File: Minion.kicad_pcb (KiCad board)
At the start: 2 copper layers, 60 x 60 mm, 70 parts, among them J1 USB_C_Receptacle_USB2.0_16P, J2 USB_A, J3 473092651, J4 PJ-320D-A, Q1 AO3401A, SW1 SW_Push, SW2 SW_Push, SW3 SW_Push, SW4 RotaryEncoder, SW5 SW_Push, SW6 SW_Push, U1 ESP32-S3-WROOM-1, U2 AMS1117-3.3, U3 FE1.1s, U4 ADXL343, U5 CH376T, U6 MCP73831-2-MC, U7 PCM5102A, Y1 12MHz, Y2 12MHz

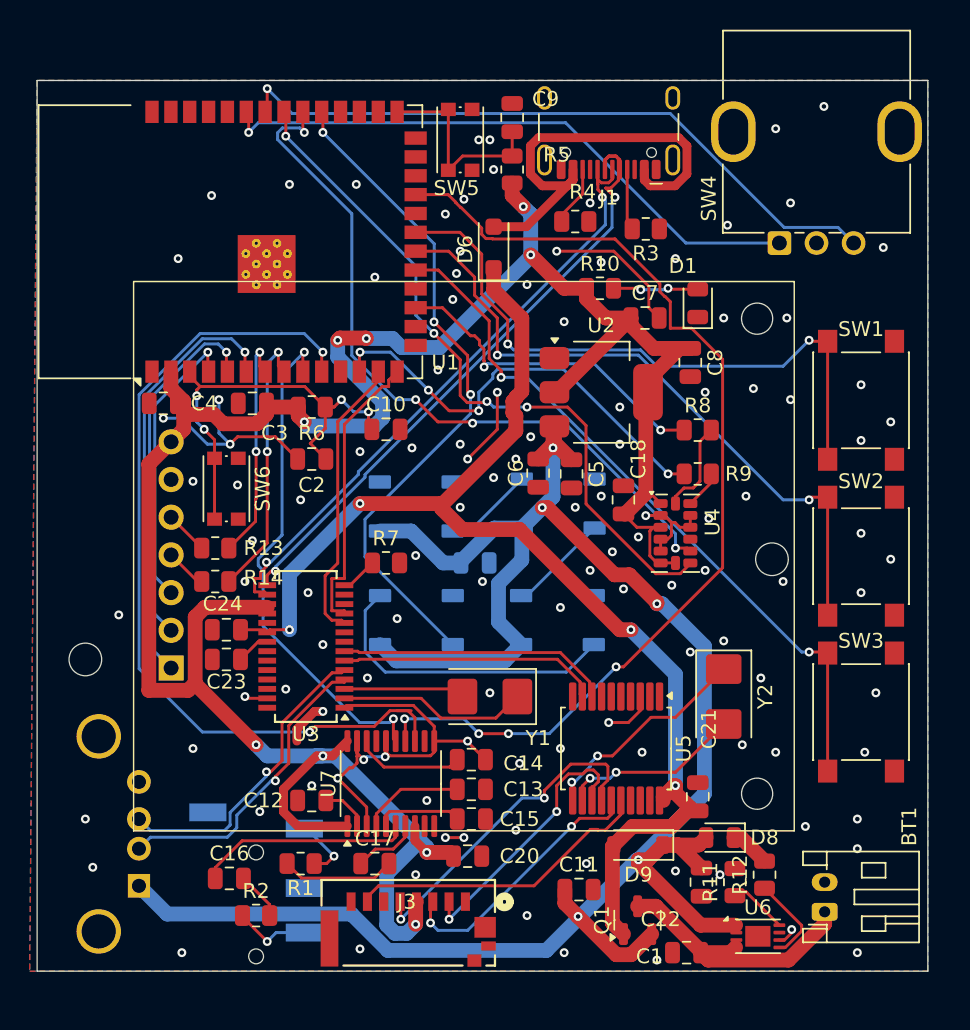
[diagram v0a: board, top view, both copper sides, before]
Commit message: Finished PCB!
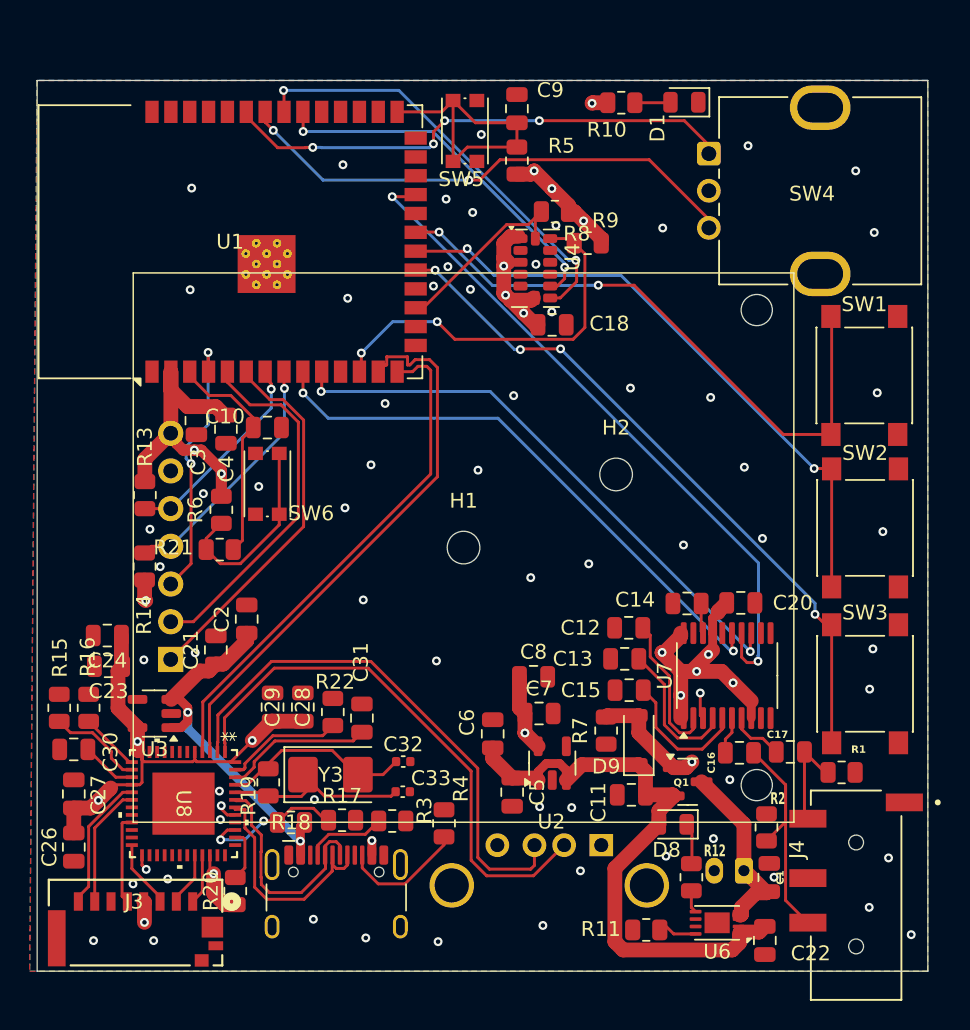
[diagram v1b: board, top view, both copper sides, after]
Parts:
- removed C19: 4.7uF, Capacitor_SMD:C_0805_2012Metric
- removed D2, D3, D4, D5: WS2812B, LED_SMD:LED_WS2812B_PLCC4_5.0x5.0mm_P3.2mm
- removed D6: S-LMBR340FT1G, Diode_SMD:D_SOD-123F
- removed DISPLAY_SSD1351: Conn_01x07_Socket, Connector_PinHeader_2.54mm:SSD_1351
- removed U5: CH376T, Package_SO:SSOP-20_5.3x7.2mm_P0.65mm
- removed Y1, Y2: 12MHz, Crystal:Crystal_SMD_5032-2Pin_5.0x3.2mm
- added C26: 0.1uF, Capacitor_SMD:C_0805_2012Metric, F.Cu at (168.5, 150.6)
- added C27: 4.7uF, Capacitor_SMD:C_0805_2012Metric, F.Cu at (168.5, 147.1)
- added C28: 4.7uF, Capacitor_SMD:C_0805_2012Metric, F.Cu at (183.9, 141.2)
- added C29: 0.1uF, Capacitor_SMD:C_0805_2012Metric, F.Cu at (181.9, 141.2)
- added C30: 0.1uF, Capacitor_SMD:C_0805_2012Metric, F.Cu at (168.5, 144.1)
- added C31: 0.1uF, Capacitor_SMD:C_0805_2012Metric, F.Cu at (187.9, 141.9)
- added C32: 18pF, Capacitor_SMD:C_0402_1005Metric, F.Cu at (190.7, 144.9)
- added C33: 18pF, Capacitor_SMD:C_0402_1005Metric, F.Cu at (190.6, 146.9)
- added J5: Conn_01x07_Socket, Connector_PinHeader_2.54mm:SSD_1351, F.Cu at (175.0, 122.8)
- added R15: 10k, Resistor_SMD:R_0805_2012Metric, F.Cu at (167.5, 141.3)
- added R16: 10k, Resistor_SMD:R_0805_2012Metric, F.Cu at (169.5, 141.3)
- added R17: 100k, Resistor_SMD:R_0805_2012Metric, F.Cu at (186.5, 148.8)
- added R18: 100k, Resistor_SMD:R_0805_2012Metric, F.Cu at (183.1, 149.0)
- added R19: 1M, Resistor_SMD:R_0805_2012Metric, F.Cu at (181.6, 146.3)
- added R20: 10k, Resistor_SMD:R_0805_2012Metric, F.Cu at (179.3, 153.6)
- added R21: 100k, Resistor_SMD:R_0805_2012Metric, F.Cu at (178.3, 130.6)
- added R22: 12k, Resistor_SMD:R_0805_2012Metric, F.Cu at (185.9, 141.5)
- added U8: USB2641I-HZH-02, USB2641:QFN48_7X7MC_MCH, F.Cu at (175.9, 147.7)
- added Y3: 24MHz, Crystal:Crystal_SMD_5032-2Pin_5.0x3.2mm, F.Cu at (185.8, 145.8)
- BT1: moved to B.Cu
- C10: value 0.1uF -> 10uF
- C2: value 1uF -> 10uF
- J4: moved to F.Cu
- R13, R14, R8, R9: value 4.7k -> 4k7
- R3, R4: value 5.1k -> 5k1
- R7: value 2.7k -> 10k
- U2: value AMS1117-3.3 -> AP2112K-3.3; footprint Package_TO_SOT_SMD:SOT-223-3_TabPin2 -> Package_TO_SOT_SMD:SOT-23-5
- U3: value FE1.1s -> AP2112K-3.3; footprint Package_SO:SSOP-28_3.9x9.9mm_P0.635mm -> Package_TO_SOT_SMD:SOT-23-5
- moved J1 56.7 mm to (186.1, 154.9), turned to 0 degrees
- moved R3 43.4 mm to (189.9, 148.9)
- moved R4 41.5 mm to (193.4, 149.0), turned to -90 degrees
- moved J4 40.4 mm to (221.2, 153.8)
- moved R1 37.0 mm to (220.2, 145.6), turned to 0 degrees
- moved C16 35.4 mm to (213.3, 144.3)
- moved R2 34.9 mm to (215.1, 149.3), turned to 90 degrees
- moved C21 33.9 mm to (178.0, 137.4)
- moved J2 31.3 mm to (204.0, 150.5), turned to 180 degrees
- moved C17 29.0 mm to (216.7, 144.2)
- moved C7 27.6 mm to (199.8, 141.6)
- moved H1 26.6 mm to (194.7, 130.5)
- moved U2 25.2 mm to (200.7, 145.0), turned to 90 degrees
- moved C20 25.1 mm to (213.4, 134.2)
- moved C12 24.3 mm to (205.8, 135.9)
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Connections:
- net BCK renamed BCK_Audio
- net IO10 renamed ROTARY_A
- net IO11 renamed ROTARY_B
- net IO12 renamed ADXL_INT1
- net IO13 renamed ADXL_INT2
- net IO4 renamed BUTTON_1
- net IO5 renamed BUTTON_2
- net IO6 renamed BUTTON_3
- net LRCK renamed LRCK_Audio
- C10 pad 1: CHIP_PU -> ESP_EN
- C2 pad 1: GND -> VUSB
- C2 pad 2: CHIP_PU -> GND
- C23 pad 1: GND -> VUSB3V3
- C23 pad 2: Net-(U3-VD33_O) -> GND
- C24 pad 1: VUSB -> VUSB3V3
- J1 pad A4: Net-(D6-A) -> VUSB
- J1 pad A9: Net-(D6-A) -> VUSB
- J1 pad B4: Net-(D6-A) -> VUSB
- J1 pad B9: Net-(D6-A) -> VUSB
- J2 pad 1: +5V -> VUSB
- J2 pad 2: D4N -> D2N
- J2 pad 3: D4P -> D2P
- J3 pad 1: unconnected-(J3-Pad1) -> SD_D2
- J3 pad 2: SCS -> SD_D3
- J3 pad 3: SDI -> SD_CMD
- J3 pad 4: +3V3 -> VUSB3V3
- J3 pad 5: SCK -> SD_CLK
- J3 pad 7: SDO -> SD_D0
- J3 pad 8: unconnected-(J3-Pad8) -> SD_D1
- J4 pad 2: Net-(J4-Pad2) -> RIGHT
- J4 pad 4: Net-(J4-Pad4) -> LEFT
- R1 pad 1: Net-(J4-Pad2) -> RIGHT
- R1 pad 2: RIGHT -> GND
- R13 pad 1: Net-(DISPLAY_SSD1351-Pin_5) -> DIN_Display
- R13 pad 2: DIN -> +3V3
- R14 pad 1: Net-(DISPLAY_SSD1351-Pin_4) -> SLK_Display
- R14 pad 2: SLK -> +3V3
- R2 pad 1: Net-(J4-Pad4) -> LEFT
- R2 pad 2: LEFT -> GND
- R6 pad 2: CHIP_PU -> Net-(R21-Pad1)
- R7 pad 1: Net-(U3-REXT) -> VUSB
- R8 pad 1: IO9/SCL -> +3V3
- R8 pad 2: Net-(U4-SCL/SCLK) -> ADXL_SCL
- R9 pad 1: IO8/SDA -> +3V3
- R9 pad 2: Net-(U4-SDA/SDI/SDIO) -> ADXL_SDA
- SW6 pad 2: CHIP_PU -> Net-(R21-Pad1)
- U1 pad 12: IO8/SDA -> ADXL_SDA
- U1 pad 17: IO9/SCL -> ADXL_SCL
- U1 pad 3: CHIP_PU -> ESP_EN
- U1 pad 31: IO14 -> Neopixels
- U1 pad 4: CS -> CS_Display
- U1 pad 5: DC -> DC_Display
- U1 pad 6: RST -> RST_Display
- U1 pad 7: DIN -> DIN_Display
- U1 pad 8: SLK -> SLK_Display
- U2 pad 1: GND -> +5V
- U2 pad 2: +3V3 -> GND
- U3 pad 1: GND -> VUSB
- U3 pad 2: Net-(U3-XOUT) -> GND
- U3 pad 3: Net-(U3-XIN) -> VUSB
- U3 pad 4: D4N -> unconnected-(U3-NC-Pad4)
- U3 pad 5: D4P -> VUSB3V3
- U4 pad 13: Net-(U4-SDA/SDI/SDIO) -> ADXL_SDA
- U4 pad 14: Net-(U4-SCL/SCLK) -> ADXL_SCL
- U7 pad 12: unconnected-(U7-SCK-Pad12) -> GND
- U7 pad 17: GND -> +3V3
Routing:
- net +3V3: track 171.5 -> 65.2 mm, vias 9 -> 16
- net +5V: track 137.8 -> 40.1 mm, vias 5 -> 0
- net GND: track 73.9 -> 1.77 mm, vias 117 -> 63
- net VUSB: track 82.6 -> 34.0 mm
- net IO14: track 45.4 -> 0.00 mm, vias 3 -> 0
- net VUSB3V3: track 0.00 -> 39.1 mm, vias 0 -> 7
- net D2N: track 0.00 -> 36.7 mm
- net D2P: track 0.00 -> 36.1 mm
- net IO8/SDA: track 29.8 -> 0.00 mm, vias 4 -> 0
- net Net-(D6-A): track 29.6 -> 0.00 mm
- net RST: track 29.1 -> 0.00 mm, vias 1 -> 0
- net CHIP_PU: track 28.9 -> 0.00 mm, vias 4 -> 0
- net DUN: track 43.6 -> 15.5 mm, vias 2 -> 0
- net DUP: track 42.3 -> 16.3 mm, vias 2 -> 0
- net ADXL_SDA: track 0.00 -> 25.8 mm, vias 0 -> 2
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- added copper zone on In2.Cu, net +3V3
- added copper zone on In1.Cu, net GND
- added copper zone on In2.Cu, net VUSB
- added copper zone on In2.Cu, net VUSB3V3
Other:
- copper layers 2 -> 4
- board text added: "-+"
